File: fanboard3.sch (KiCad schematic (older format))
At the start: 27 parts, among them J1 PWR IN, J10 Conn_01x14_Male, J11 USB_A, J12 Conn_01x02_Male, J2 Conn_02x08_Odd_Even, J6 FAN1, J7 FAN2, J8 FAN3, J9 FAN4, K1 G6K-2, M1 5V, M2 12V, P1 Conn_02x20_Odd_Even, Q1 2SD1047, U1 SN74HCT245

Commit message: added Volt meter and changed layout
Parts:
- removed J10: Conn_01x14_Male, Connectors_Phoenix:PhoenixContact_MCV-G_14x3.81mm_Vertical, symbol Connector:Conn_01x14_Male
- added J3: Conn_01x10_Male, Connectors_Phoenix:PhoenixContact_MCV-G_10x3.81mm_Vertical, symbol Connector:Conn_01x10_Male
- added R10, R12, R8: 10K, Resistors_SMD:R_1210_HandSoldering, symbol Device:R
- added R11, R7, R9: 100K, Resistors_SMD:R_1210_HandSoldering, symbol Device:R
- added U2: MCP3008, Housings_SSOP:SOP-16_4.4x10.4mm_Pitch1.27mm, symbol Analog_ADC:MCP3008
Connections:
- net labels added: B1, B2, B3, B4, FAN1-PWM, FAN1-RPM, FAN2-PWM, FAN2-RPM, FAN3-PWM, FAN3-RPM, FAN4-PWM, FAN4-RPM, GPI010, GPIO17, GPIO18, MISO, MOSI, PWM0, PWM0-5V, PWM1, PWM1-5V, SCLK
- net labels removed: 12V, 5V
- wire segments 271 -> 174
- no-connect marks 29 -> 28
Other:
- moved on the sheet: D1, D2, J1, J11, J2, J6, J7, J8, J9, K1, M1A, M2A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

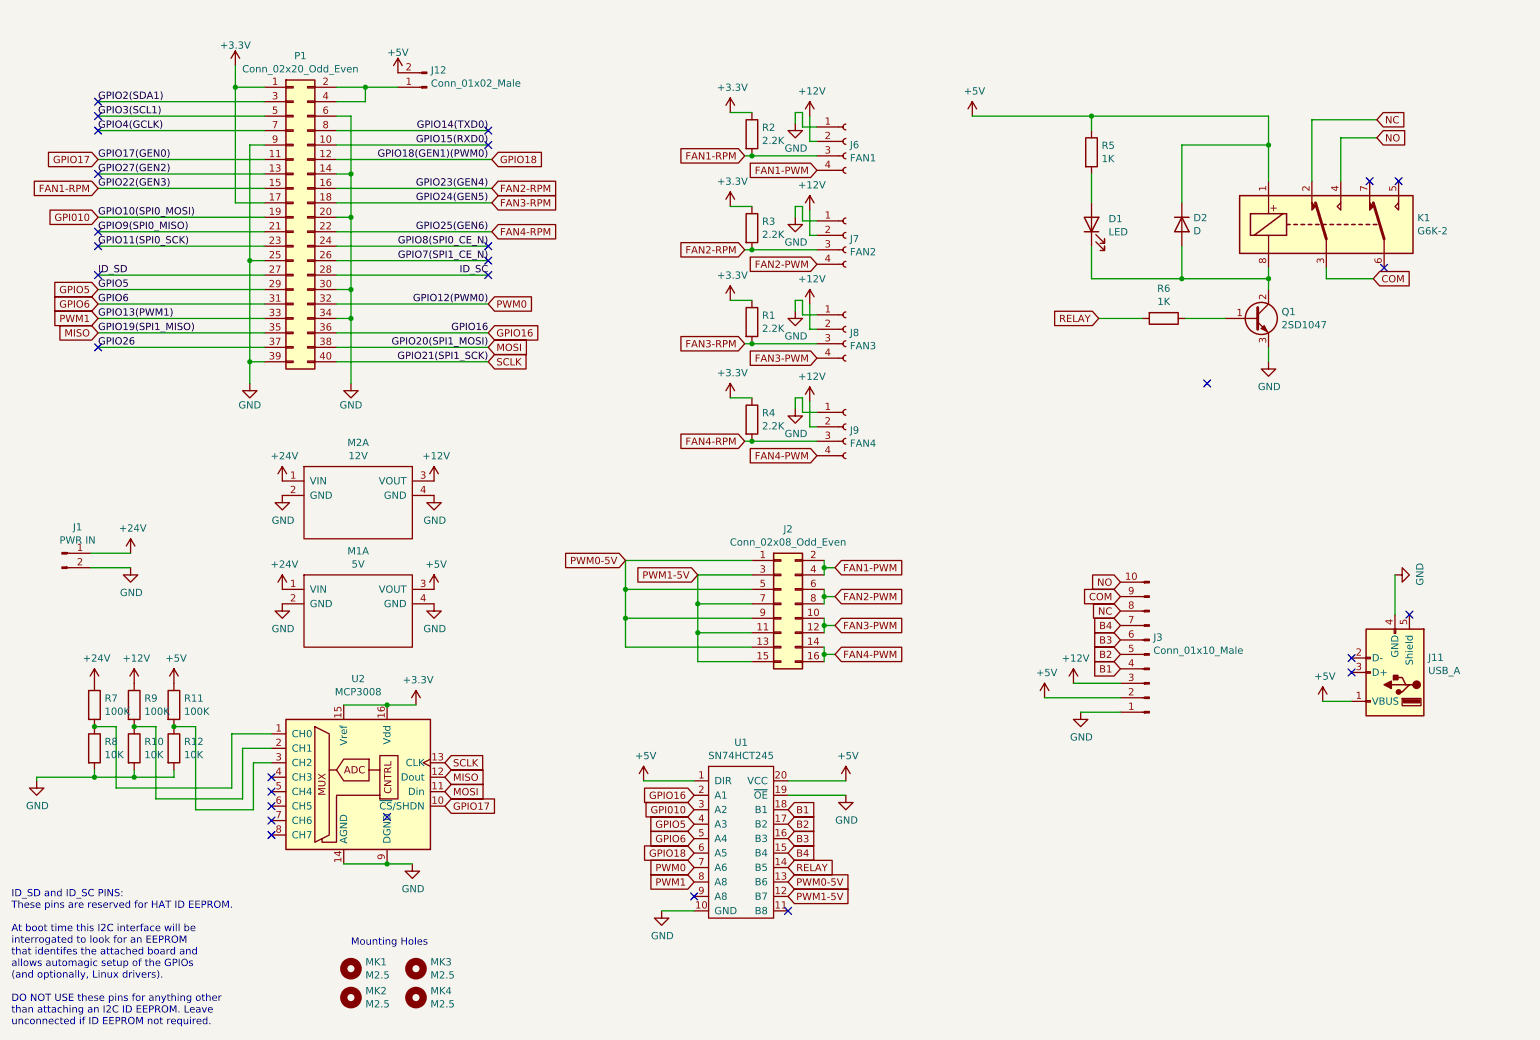
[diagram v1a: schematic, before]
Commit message: Updates
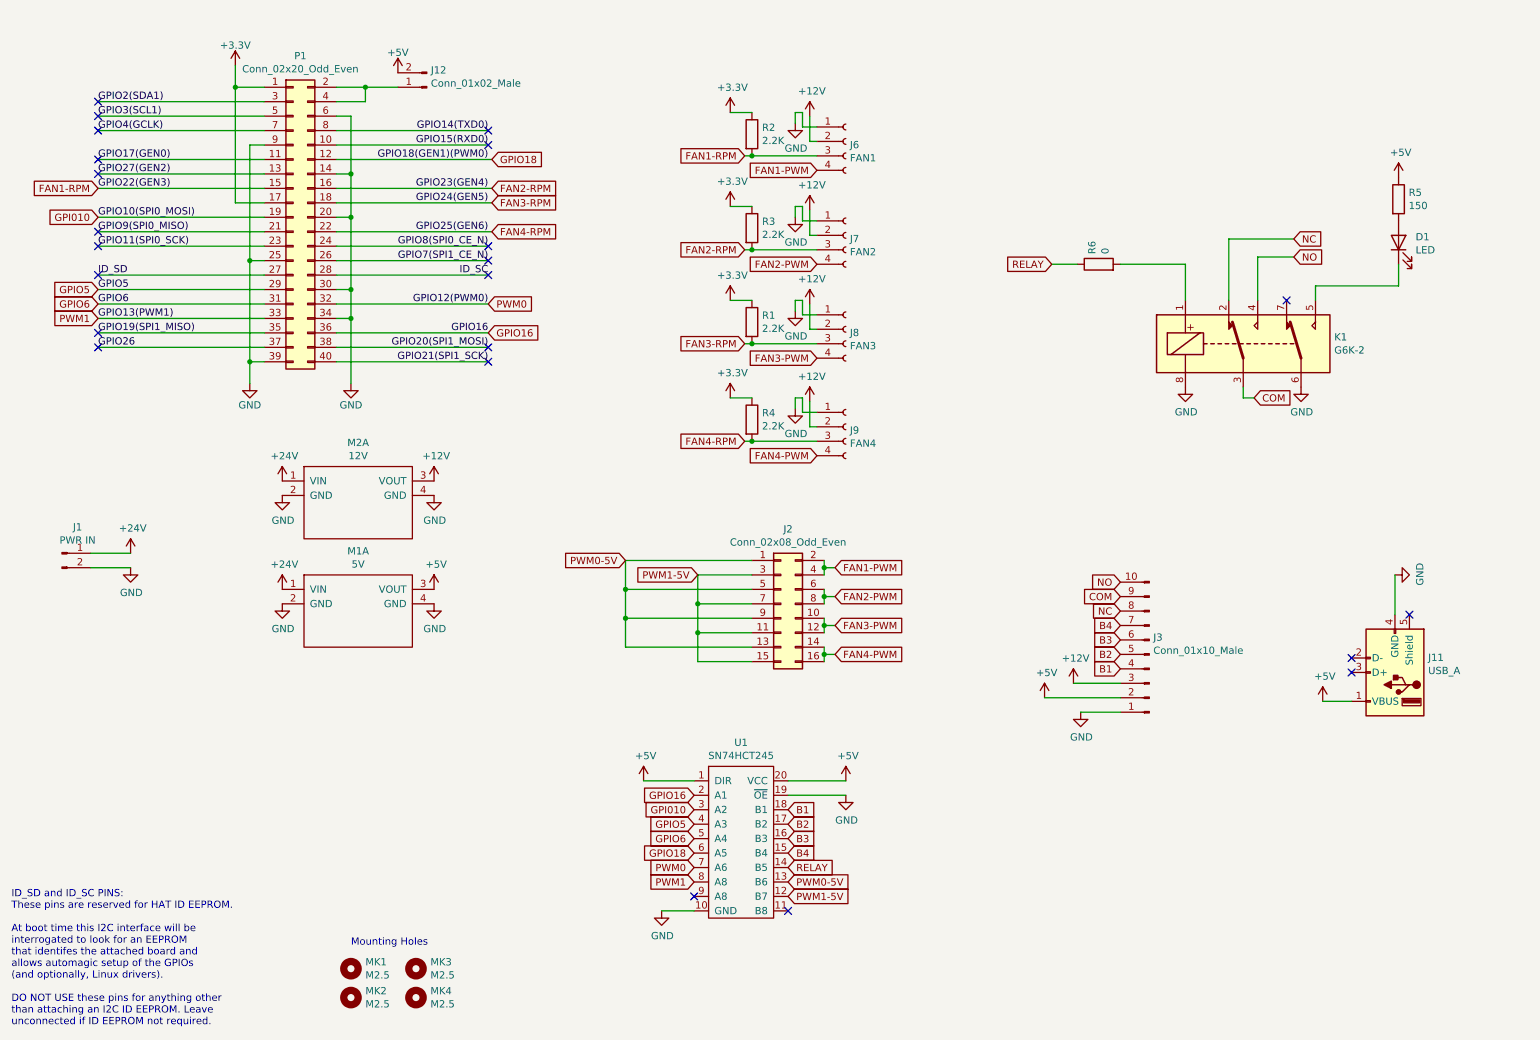
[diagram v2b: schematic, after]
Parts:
- removed D2: D, Diodes_SMD:D_SMA, symbol Device:D
- removed Q1: 2SD1047, TO_SOT_Packages_SMD:SOT-223, symbol Transistor_BJT:2SD1047
- removed R10, R12, R8: 10K, Resistors_SMD:R_1210_HandSoldering, symbol Device:R
- removed R11, R7, R9: 100K, Resistors_SMD:R_1210_HandSoldering, symbol Device:R
- removed U2: MCP3008, Housings_SSOP:SOP-16_4.4x10.4mm_Pitch1.27mm, symbol Analog_ADC:MCP3008
- R5: value 1K -> 150
- R6: value 1K -> 0
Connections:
- net +5V: no longer K1.1
- net GND: now also K1.6, K1.8
- net RELAY: now also R6.1; no longer R6.2
- net at D1.1 (K): now also K1.5; no longer K1.8
- net GPIO17 renamed GPIO17(GEN0)
- net MISO renamed GPIO19(SPI1_MISO)
- net MOSI renamed GPIO20(SPI1_MOSI)
- net SCLK renamed GPIO21(SPI1_SCK)
- new net: K1.1, R6.2
- no-connect marks 28 -> 23
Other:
- moved on the sheet: D1, K1, R5
